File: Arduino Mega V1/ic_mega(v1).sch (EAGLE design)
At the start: 45 parts, among them IC1 TL071P, IC2 LM7805, J1 F-2X07-79107_M, J5 F-1X02-SIP-100-32, J6 DAC, U2 INA333AIDRGT, U3 INA333AIDRGT, U4 INA333AIDRGT, U5 INA333AIDRGT

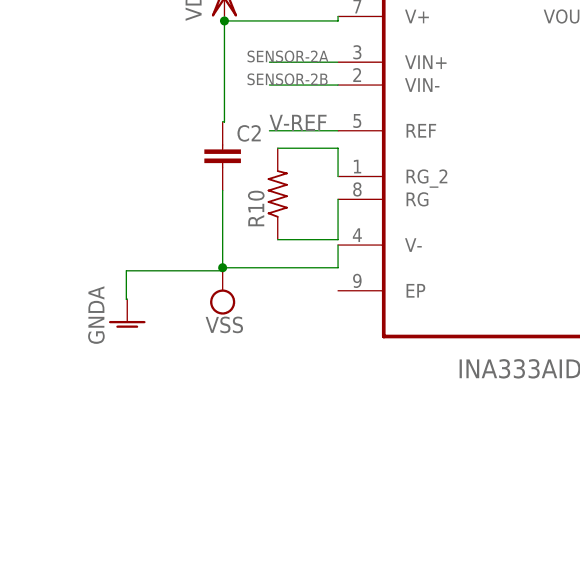
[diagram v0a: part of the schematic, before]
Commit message: versao final 1
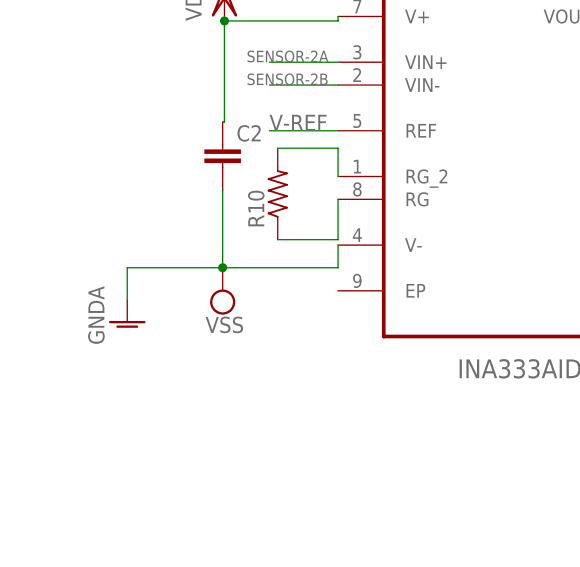
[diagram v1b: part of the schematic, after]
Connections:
- net GNDA: now also C2.2, U3.V-
- net VSS: no longer C2.2, U3.V-
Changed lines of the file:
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@@
 <label x="353" y="86.6" size="1.778" layer="95"/>
+</segment>
+<segment>
+<pinref part="C2" gate="G$1" pin="2"/>
+<pinref part="SUPPLY4" gate="G$1" pin="VSS"/>
+<wire x1="32.9" y1="54.32" x2="32.9" y2="45.74" width="0.1524" layer="91"/>
+<wire x1="32.9" y1="45.74" x2="32.9" y2="45.4" width="0.1524" layer="91"/>
+<junction x="32.9" y="45.74"/>
+<pinref part="U3" gate="A" pin="V-"/>
+<wire x1="45.72" y1="48.26" x2="45.72" y2="45.74" width="0.1524" layer="91"/>
+<wire x1="45.72" y1="45.74" x2="32.9" y2="45.74" width="0.1524" layer="91"/>
+<pinref part="GND5" gate="1" pin="GNDA"/>
+<wire x1="22.3" y1="42.24" x2="22.3" y2="45.74" width="0.1524" layer="91"/>
+<wire x1="22.3" y1="45.74" x2="32.9" y2="45.74" width="0.1524" layer="91"/>
 </segment>
 </net>
@@
 </segment>
 <segment>
-<pinref part="C2" gate="G$1" pin="2"/>
-<pinref part="SUPPLY4" gate="G$1" pin="VSS"/>
-<wire x1="32.9" y1="54.32" x2="32.9" y2="45.74" width="0.1524" layer="91"/>
-<wire x1="32.9" y1="45.74" x2="32.9" y2="45.4" width="0.1524" layer="91"/>
-<wire x1="32.9" y1="45.4" x2="22.2" y2="45.4" width="0.1524" layer="91"/>
-<junction x="32.9" y="45.74"/>
-<pinref part="GND5" gate="1" pin="GNDA"/>
-<wire x1="22.2" y1="45.4" x2="22.2" y2="42.24" width="0.1524" layer="91"/>
-<wire x1="22.2" y1="42.24" x2="22.3" y2="42.24" width="0.1524" layer="91"/>
-<pinref part="U3" gate="A" pin="V-"/>
-<wire x1="45.72" y1="48.26" x2="45.72" y2="45.74" width="0.1524" layer="91"/>
-<wire x1="45.72" y1="45.74" x2="32.9" y2="45.74" width="0.1524" layer="91"/>
-</segment>
-<segment>
